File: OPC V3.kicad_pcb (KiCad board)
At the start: 4 copper layers, 65 x 43 mm, 57 parts, among them J1 691382010004, J2 691382010004, J3 MEC1-110-02-F-D-A, J4 691382010004, J5 Conn_01x05, J6 Conn_01x04_Pin, U1 TS3A4751PWR, U2 TS3A4751PWR, U3 MCP23017x-x-ML, U4 TS3A4751PWR, U5 ADS1120-PW, U6 TS3A4751PWR, U7 BMP581, U8 DS3231MZ, U9 TS3A4751PWR

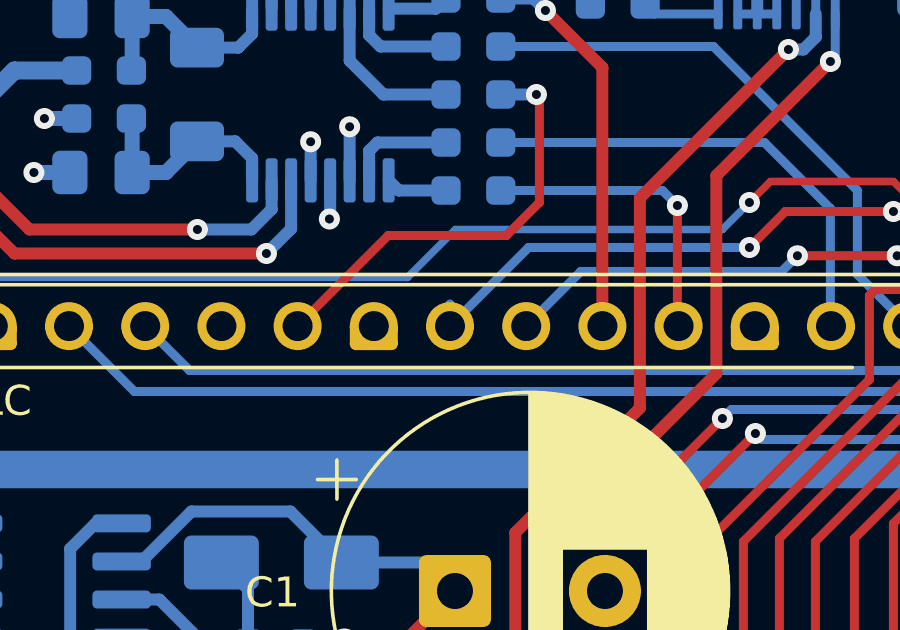
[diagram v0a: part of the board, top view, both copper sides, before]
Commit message: MAJ post prod
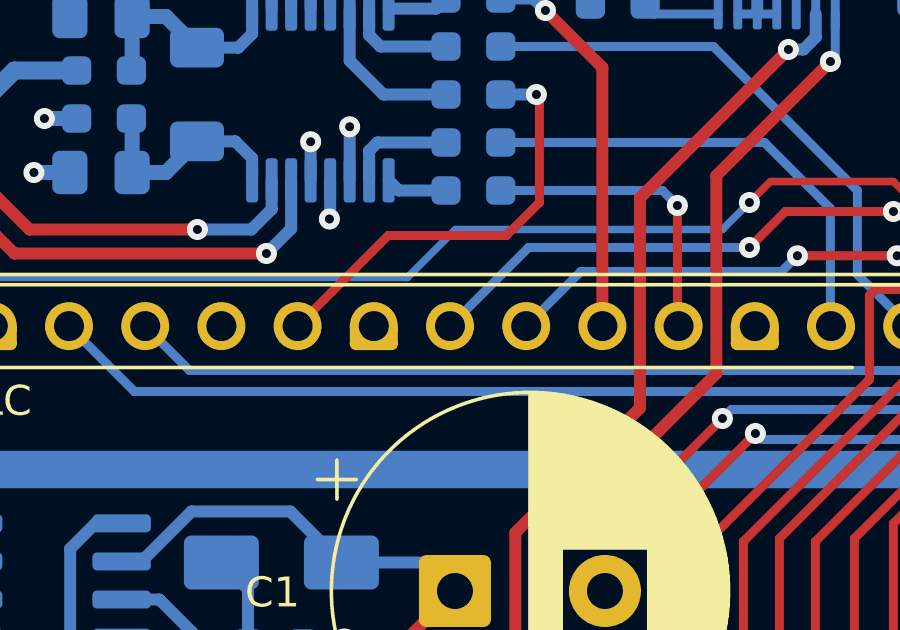
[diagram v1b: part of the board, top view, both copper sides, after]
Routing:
- net /Connecteur/OUTPUT_1: track 25.6 -> 24.8 mm
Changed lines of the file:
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@@
-	)
-	(segment
-		(start 148.02 122.22)
-		(end 148.02 121.48)
-		(width 0.3)
-		(layer "B.Cu")
-		(net "/Connecteur/OUTPUT_1")
 	)
 	(segment
